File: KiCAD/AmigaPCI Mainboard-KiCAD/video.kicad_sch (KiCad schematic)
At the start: 37 parts, among them CN300 DB15_Female_HighDensity, CN301 Video-Slot, CN302 Video-Slot, J303 HSYNC/COMPSYNC, U300 DENISE, U301 74AHCT244, U302 74AHCT244, U305 74HCT08

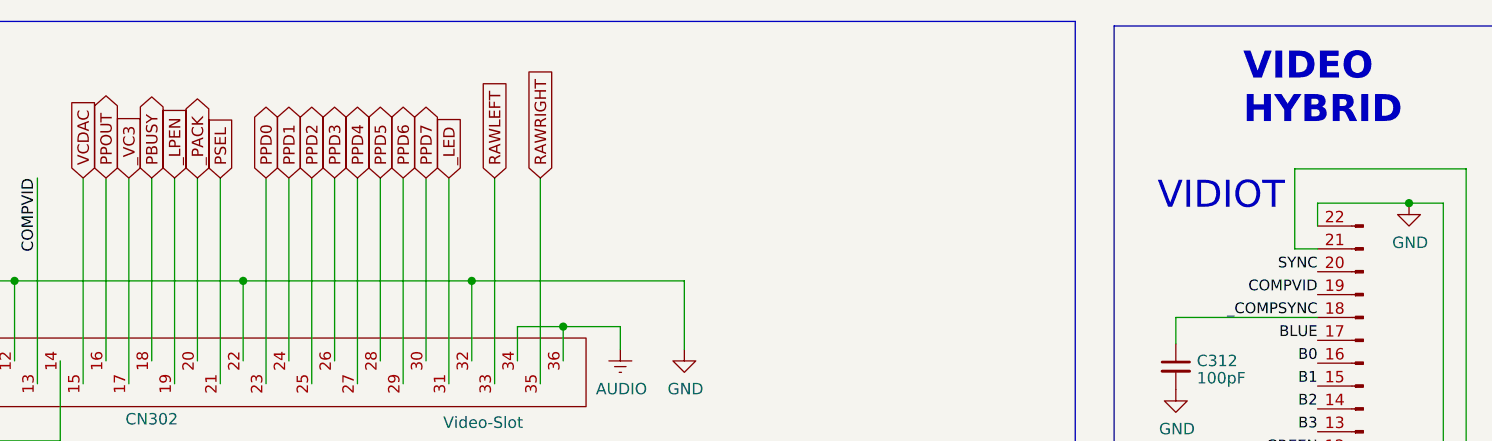
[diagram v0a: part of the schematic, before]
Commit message: Updated Schematic 12-DEC-2023
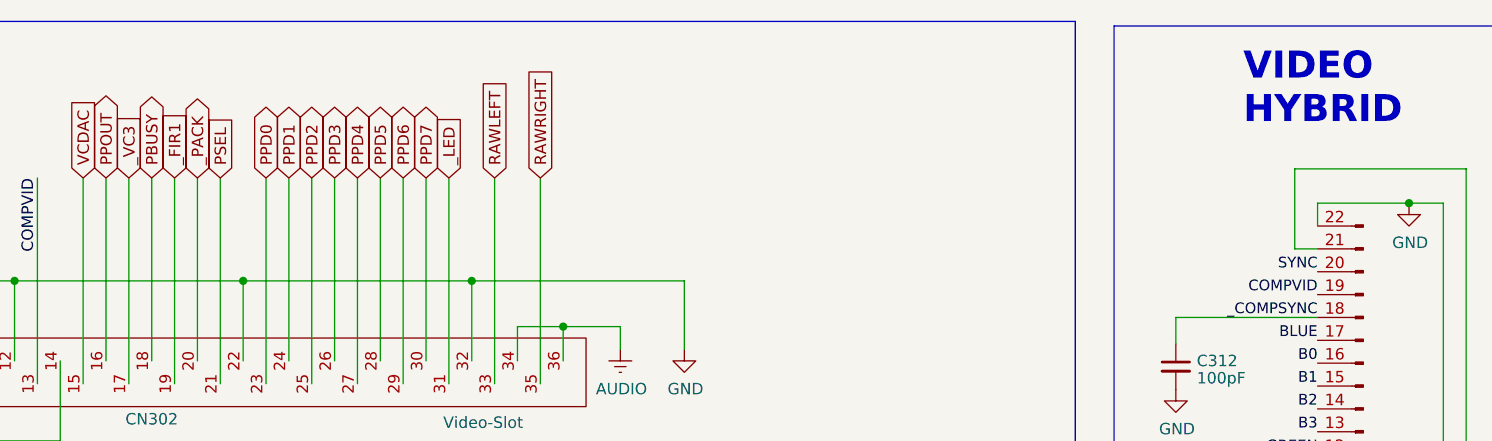
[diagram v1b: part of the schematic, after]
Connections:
- net _LPEN renamed _FIR1
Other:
- note removed: "VIDIOT"
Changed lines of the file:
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@@
     (effects (font (size 6 6) (thickness 1.2) bold) (justify left bottom))
-  )
-  (text "VIDIOT" (at 366.268 35.306 0)
-    (effects (font (size 2.9972 2.9972)) (justify left bottom))
   )
   (label "DRD4" (at 47.625 85.344 180) (fields_autoplaced)
@@
     )
   )
-  (global_label "_LPEN" (shape input) (at 257.048 31.496 90) (fields_autoplaced)
-    (effects (font (size 1.27 1.27)) (justify left))
-    (property "Intersheetrefs" "${INTERSHEET_REFS}" (at 257.048 22.845 90)
-      (effects (font (size 1.27 1.27)) (justify left))
-    )
+  (global_label "_FIR1" (shape input) (at 257.048 31.496 90) (fields_autoplaced)
+    (effects (font (size 1.27 1.27)) (justify left))
+    (property "Intersheetrefs" "${INTERSHEET_REFS}" (at 257.048 23.3703 90)
+      (effects (font (size 1.27 1.27)) (justify left))
+    )

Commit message: Schematic and PCB Updates 13-DEC-2023
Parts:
- removed RN300: 1k, Resistor_THT:R_Array_SIP6, symbol Device:R_Network05
- added R303, R309, R311, R312: 1k, Resistor_SMD:R_0603_1608Metric, symbol Device:R_Small
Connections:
- net GND: now also R303.1, R309.1, R311.1, R312.1
- net M0H: now also R311.2
- net M0V: now also R309.2
- net M1H: now also R303.2
- net M1V: now also R312.2
- net 7M renamed CLK7
- no-connect marks 10 -> 9
